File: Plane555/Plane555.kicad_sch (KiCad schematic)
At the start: 10 parts, among them SW1 SW_SPDT, U1 LM555xM

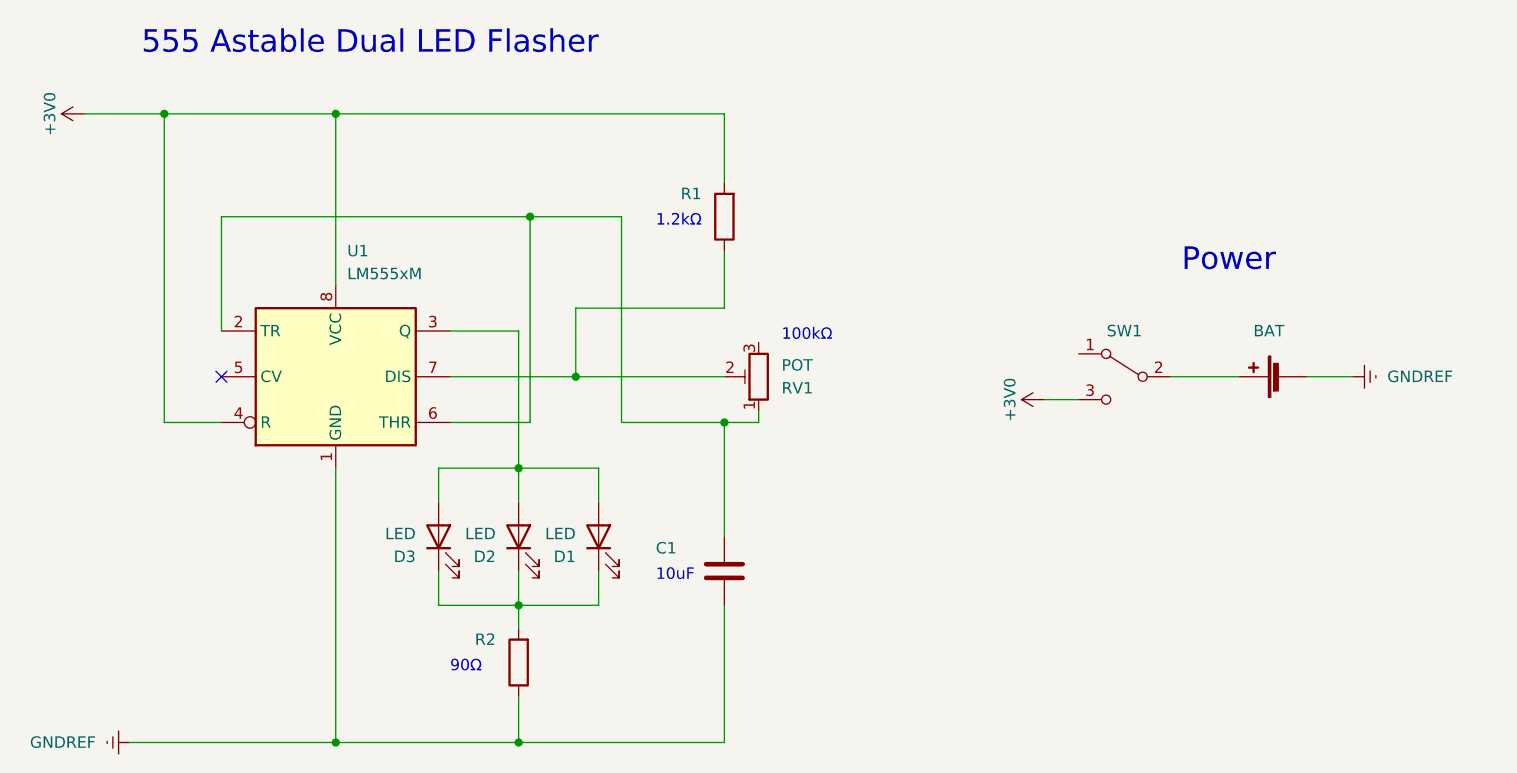
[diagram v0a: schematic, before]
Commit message: feat: init new files
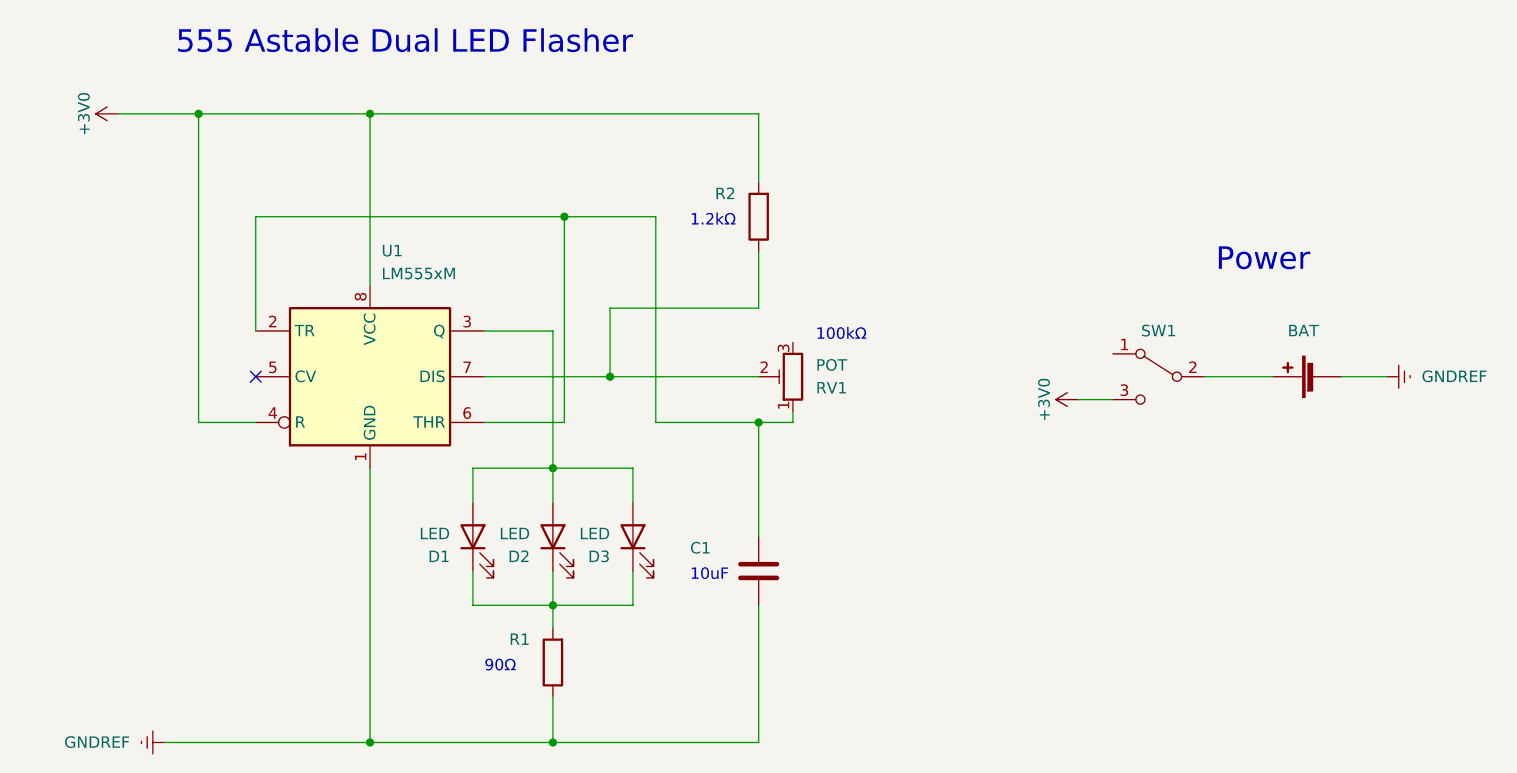
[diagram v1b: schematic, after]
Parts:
- D1: footprint LED_THT:LED_D3.0mm -> LED_THT:LED_D3.0mm_Horizontal_O1.27mm_Z2.0mm
- D3: footprint LED_THT:LED_D3.0mm_Horizontal_O1.27mm_Z2.0mm -> LED_THT:LED_D3.0mm
- SW1: footprint SW SS12D:Schiebeschalter SS-12D00.kicad_mod -> Button_Switch_THT:Schiebeschalter_SS-12D00
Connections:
- net +3V0: now also R2.2; no longer R1.2
- net GNDREF: now also R1.1; no longer R2.1
- net at RV1.2, U1.7 (DIS): now also R2.1; no longer R1.1
- net at D1.1 (K), D2.1 (K), D3.1 (K): now also R1.2; no longer R2.2
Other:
- title: 555 Airplane PCB with Dual Flashing LED -> Plane 555 Astable Dual LED Flasher 
